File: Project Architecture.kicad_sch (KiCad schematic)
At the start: 0 parts

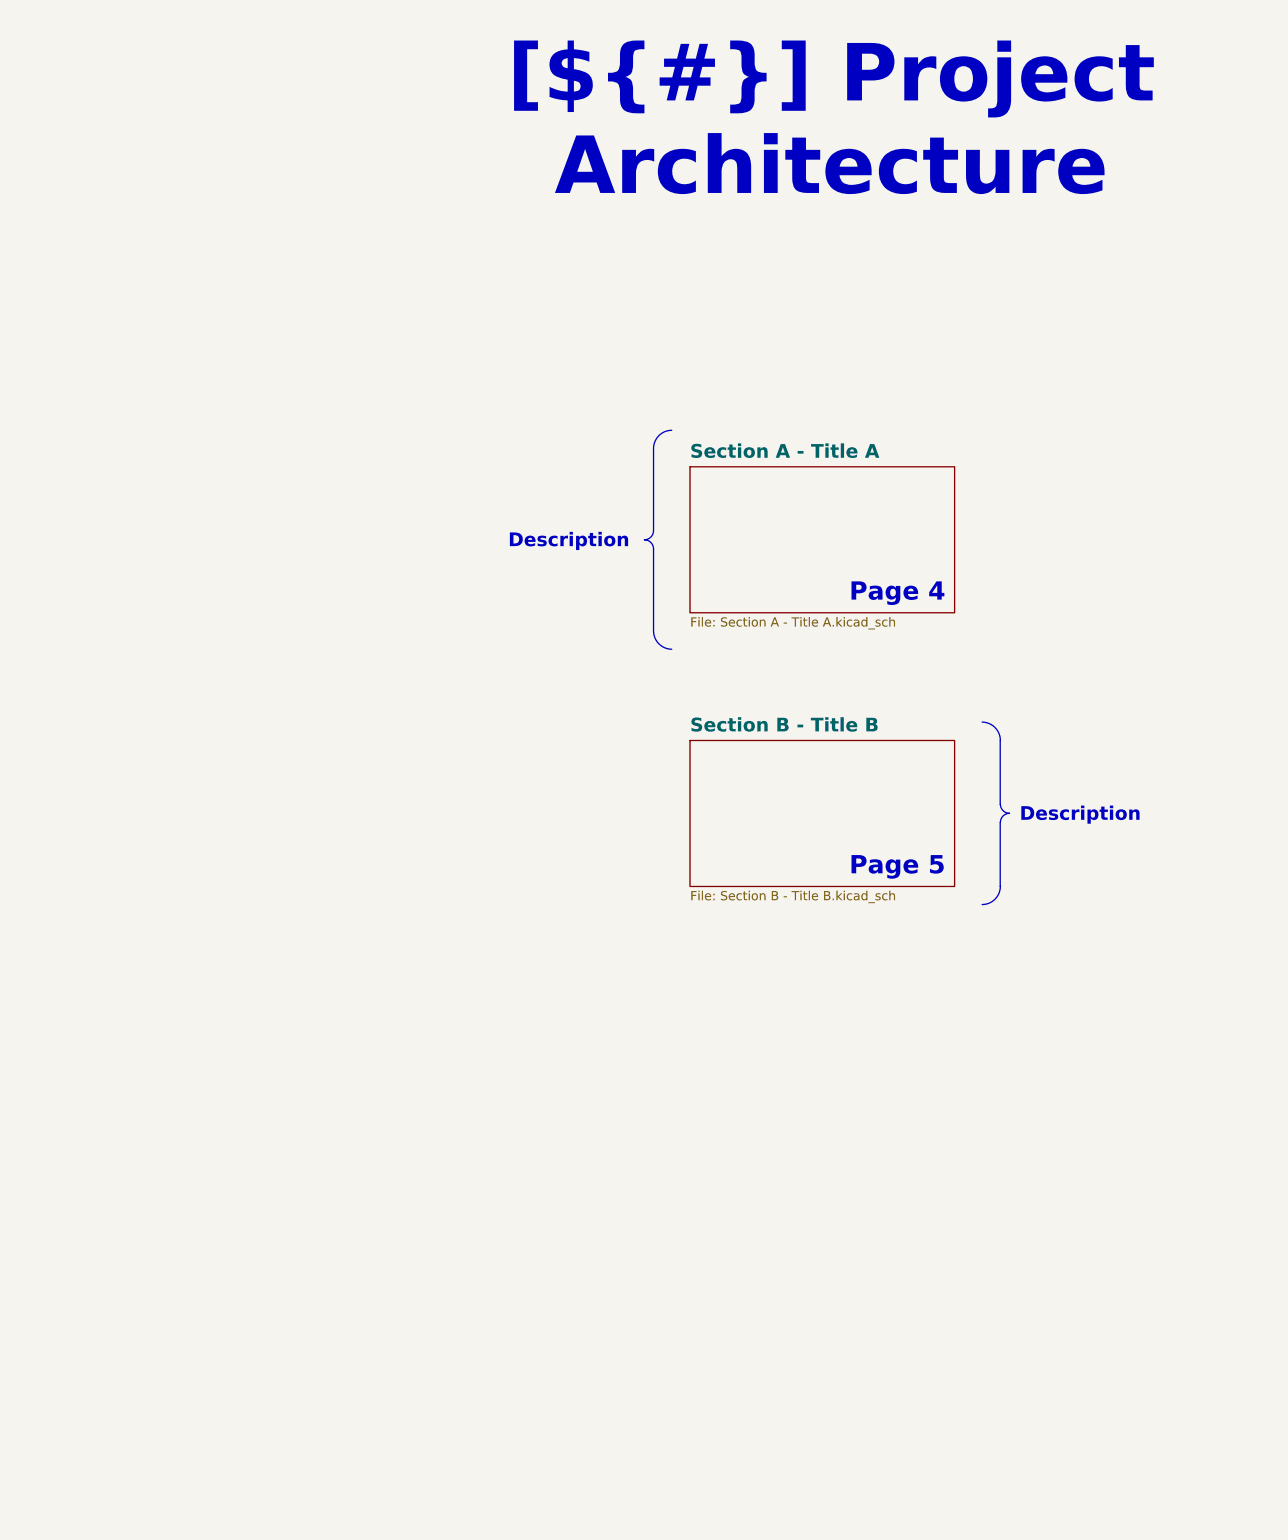
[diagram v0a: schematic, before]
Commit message: SCH[Power & Balance]: Inital Schamtic for two pages.
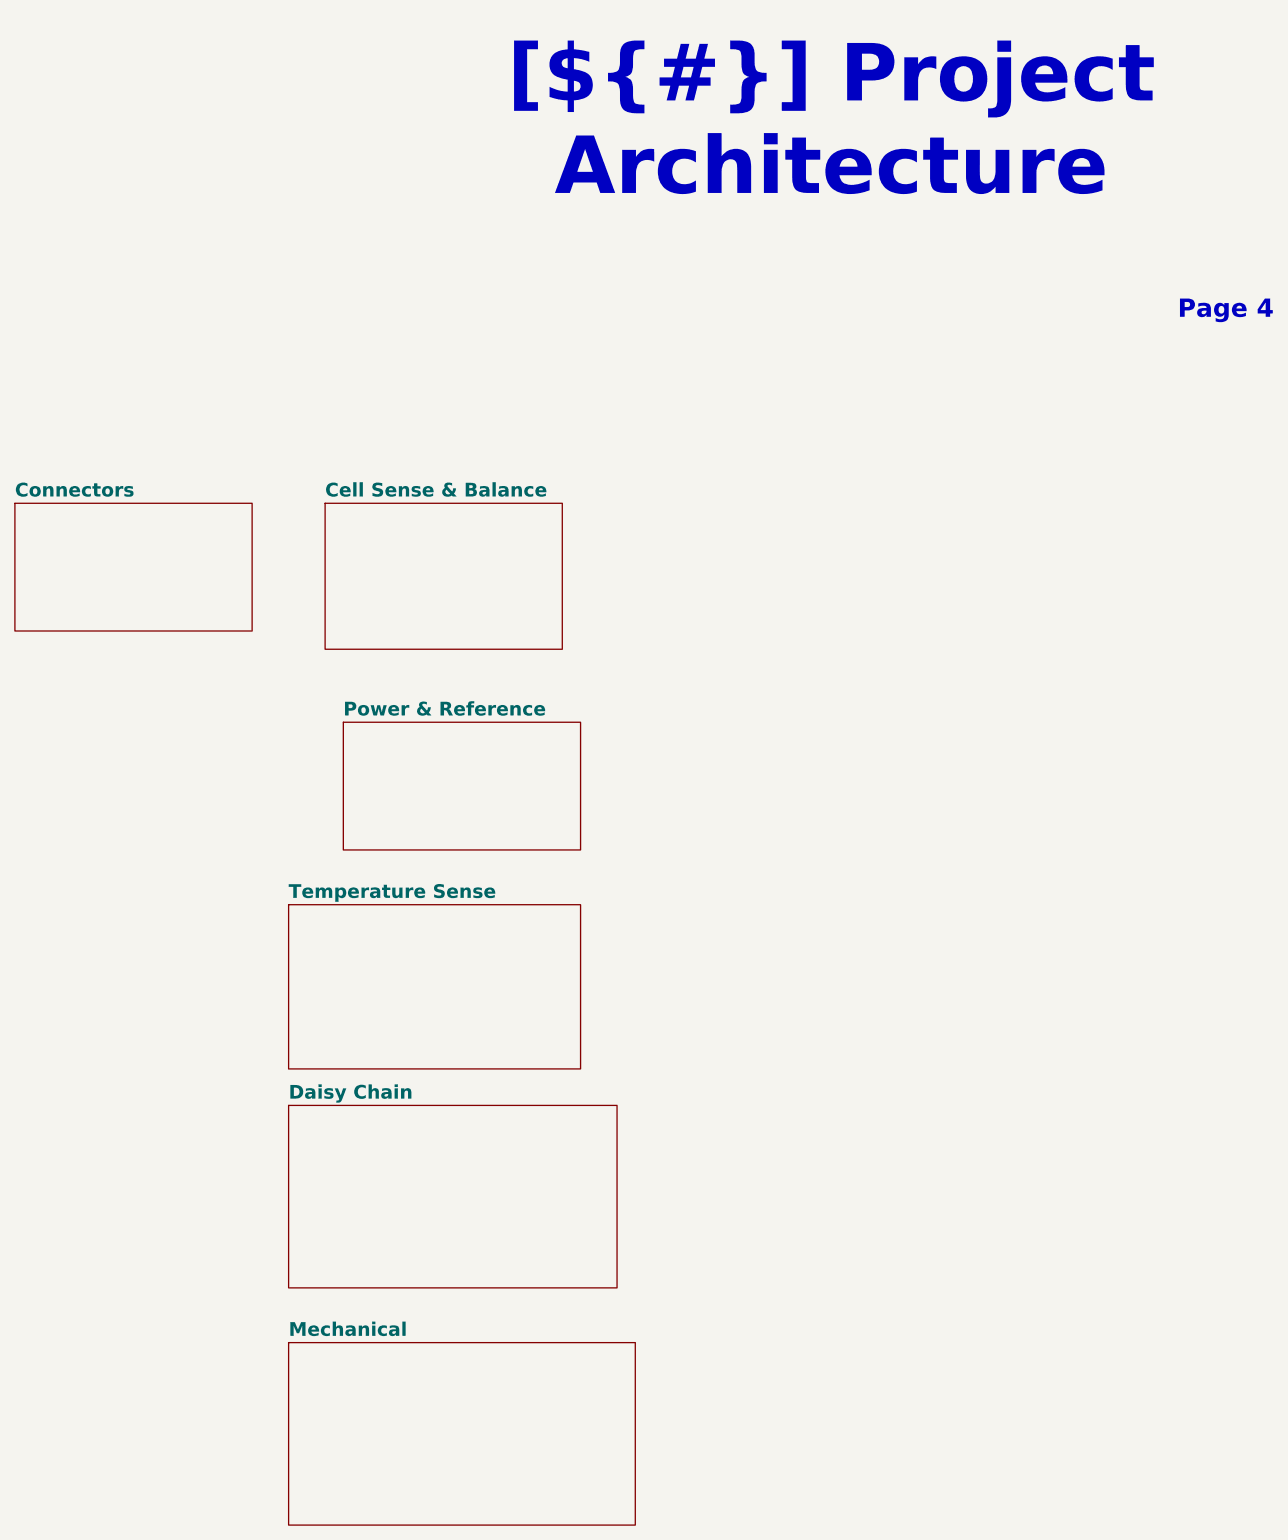
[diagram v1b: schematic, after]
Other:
- removed sheet Section A - Title A
- removed sheet Section B - Title B
- added sheet Cell Sense & Balance (cell_sense_and_balance.kicad_sch)
- added sheet Connectors (connectors.kicad_sch)
- added sheet Daisy Chain (daisy_chain.kicad_sch)
- added sheet Mechanical (mechanical.kicad_sch)
- added sheet Power & Reference (power_and_reference.kicad_sch)
- added sheet Temperature Sense (temperature_sense.kicad_sch)
- note removed: "Page 5"
